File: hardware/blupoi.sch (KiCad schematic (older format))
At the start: 19 parts, among them P1 MICRO-B-USB, P2 CONN_02X05, P3 SERIAL, U1 NRF52832, X1 32MHz

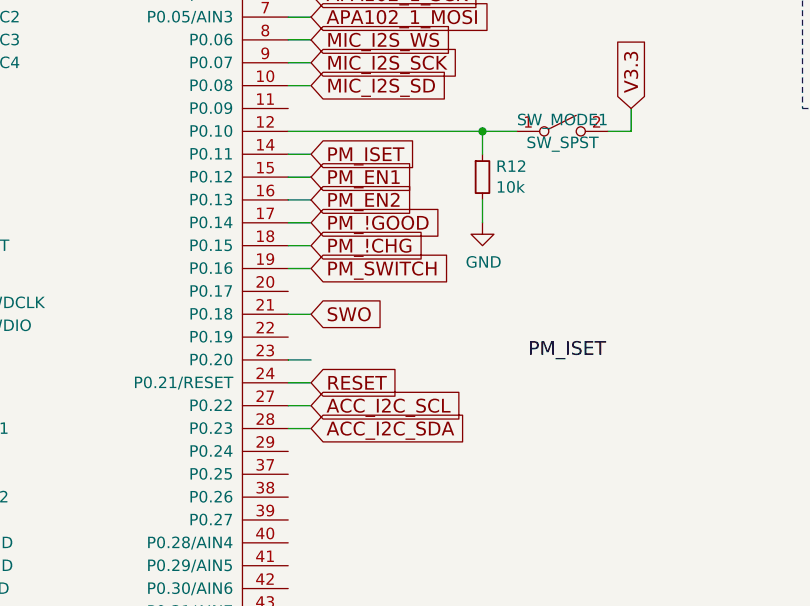
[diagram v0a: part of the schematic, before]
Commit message: Finished routing for v0.2
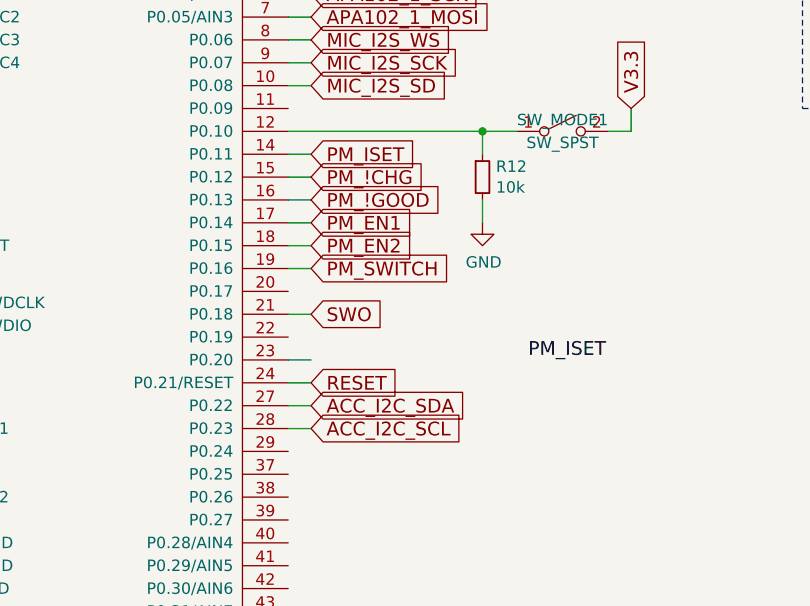
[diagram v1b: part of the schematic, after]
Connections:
- net ACC_I2C_SCL: now also U1.28 (P0.23); no longer U1.27 (P0.22)
- net ACC_I2C_SDA: now also U1.27 (P0.22); no longer U1.28 (P0.23)
- net PM_!CHG: now also U1.15 (P0.12); no longer U1.18 (P0.15)
- net PM_!GOOD: now also U1.16 (P0.13); no longer U1.17 (P0.14)
- net PM_EN1: now also U1.17 (P0.14); no longer U1.15 (P0.12)
- net PM_EN2: now also U1.18 (P0.15); no longer U1.16 (P0.13)
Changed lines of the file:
@@
 Text GLabel 6800 2300 2    60   Input ~ 0
 MIC_I2S_SD
+Text GLabel 6800 3800 2    60   Input ~ 0
+ACC_I2C_SCL
 Text GLabel 6800 3700 2    60   Input ~ 0
-ACC_I2C_SCL
-Text GLabel 6800 3800 2    60   Input ~ 0
 ACC_I2C_SDA
 Text GLabel 10350 1400 2    60   Input ~ 0
@@
 Text GLabel 6800 2600 2    60   Input ~ 0
 PM_ISET
+Text GLabel 6800 2900 2    60   Input ~ 0
+PM_EN1
+Text GLabel 6800 3000 2    60   Input ~ 0
+PM_EN2
+Text GLabel 6800 2800 2    60   Input ~ 0
+PM_!GOOD
 Text GLabel 6800 2700 2    60   Input ~ 0
-PM_EN1
-Text GLabel 6800 2800 2    60   Input ~ 0
-PM_EN2
-Text GLabel 6800 2900 2    60   Input ~ 0
-PM_!GOOD
-Text GLabel 6800 3000 2    60   Input ~ 0
 PM_!CHG
 Text GLabel 6800 3100 2    60   Input ~ 0
